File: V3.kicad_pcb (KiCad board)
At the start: 2 copper layers, 164.6 x 93.3 mm, 73 parts, among them IC1 MCP4451-103E_ST, IC2 MCP4451-103E_ST, IC3 MCP4451-103E_ST, IC4 MCP4451-103E_ST, IC5 MCP4451-103E_ST, IC6 MCP4451-103E_ST, J1 Barrel_Jack, J2 Conn_01x22_Female, U1 AMPLIFIER-PAM8403, U10 AMPLIFIER-PAM8403, U11 AMPLIFIER-PAM8403, U12 AMPLIFIER-PAM8403, U2 AMPLIFIER-PAM8403, U3 AMPLIFIER-PAM8403, U4 AMPLIFIER-PAM8403, U5 AMPLIFIER-PAM8403, U6 AMPLIFIER-PAM8403, U7 AMPLIFIER-PAM8403, U8 AMPLIFIER-PAM8403, U9 AMPLIFIER-PAM8403

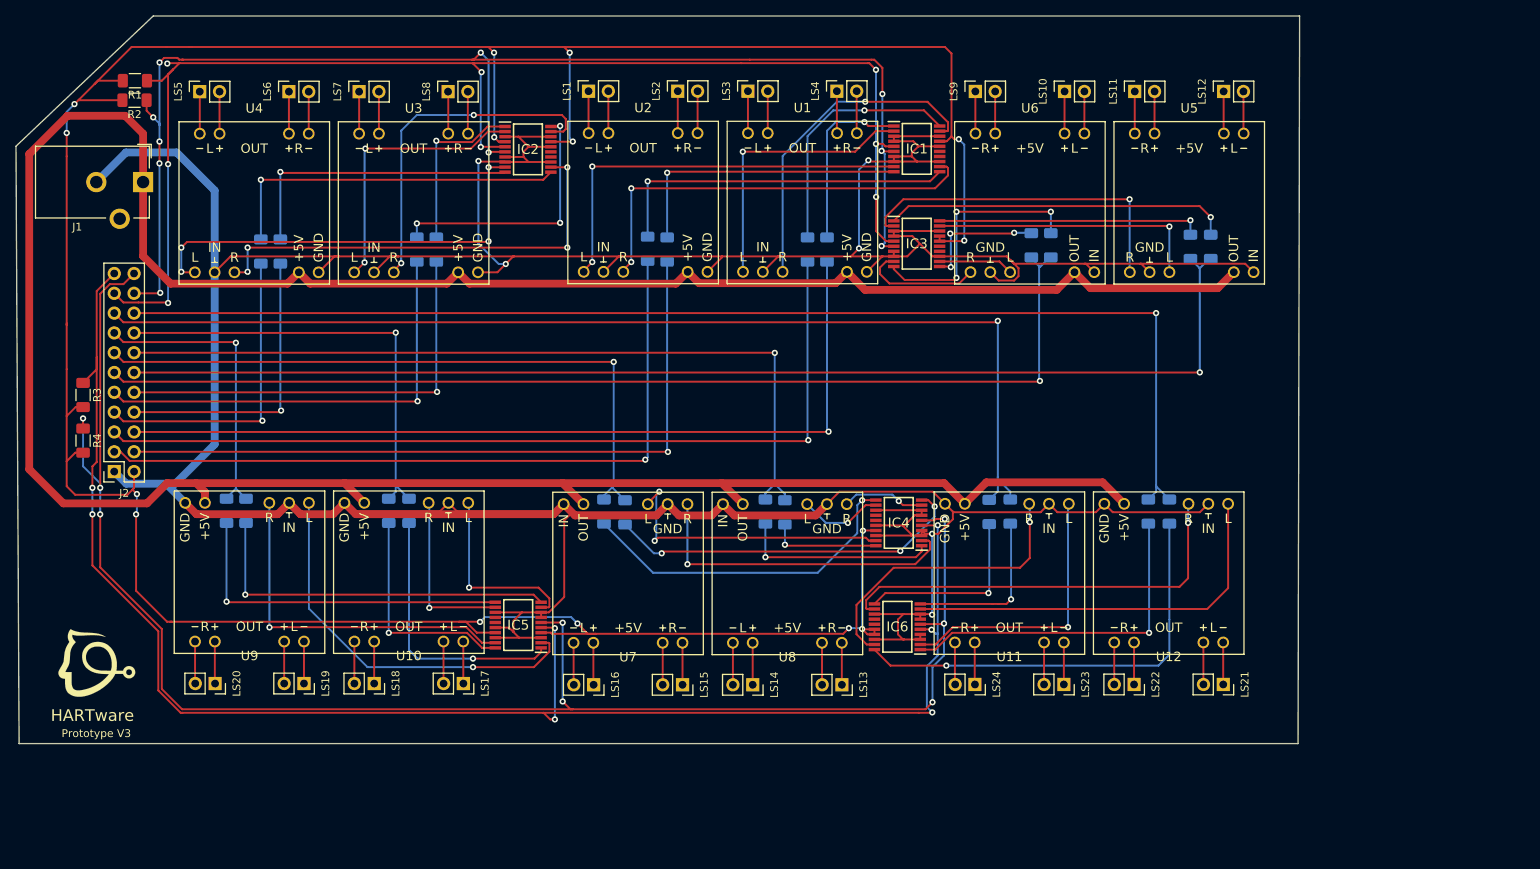
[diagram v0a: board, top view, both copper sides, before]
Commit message: Release V3.0.1
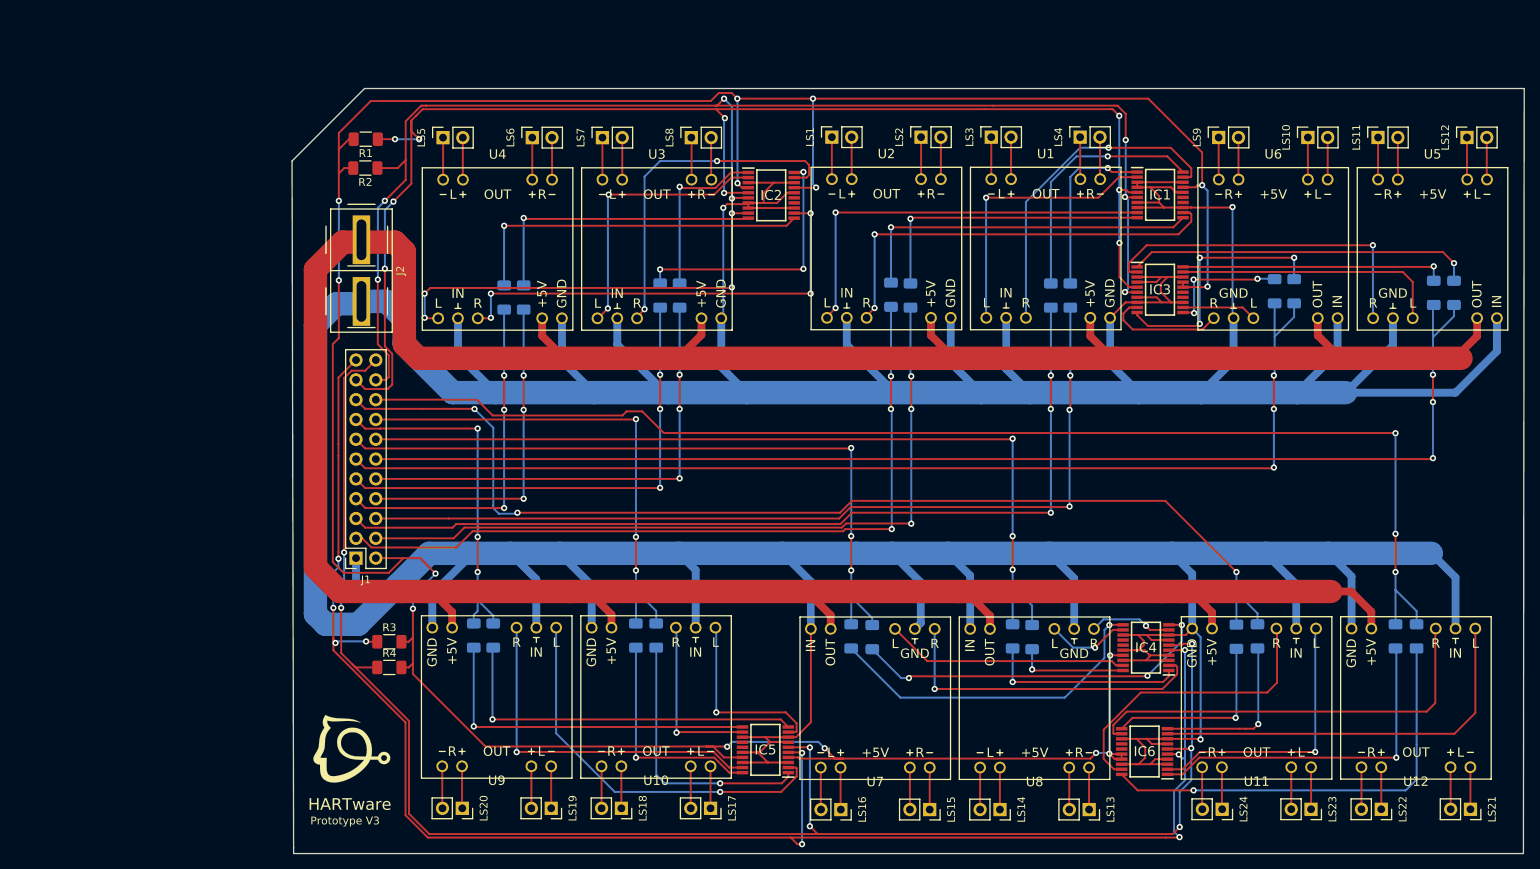
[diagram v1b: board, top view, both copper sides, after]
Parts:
- J1: value Barrel_Jack -> Conn_01x22_Female; footprint Barrel Jack:BarrelJack_CUI_PJ-102AH_Horizontal -> Pin Socket 2.54mm:PinSocket_2x11_P2.54mm_Vertical
- J2: value Conn_01x22_Female -> PowerPole; footprint Pin Socket 2.54mm:PinSocket_2x11_P2.54mm_Vertical -> PowerPole:45A-VERT-PAIR
- moved J1 55.4 mm to (128.8, 118.9), turned to 180 degrees
- moved R3 50.4 mm to (133.1, 129.6), turned to 0 degrees
- moved R4 48.9 mm to (133.1, 132.9), turned to 0 degrees
- moved J2 40.9 mm to (129.5, 82.0), turned to 270 degrees
- moved IC5 35.5 mm to (181.3, 143.5)
- moved LS14 35.5 mm to (211.4, 151.2)
- moved LS15 35.5 mm to (202.4, 151.2)
- moved LS17 35.5 mm to (174.3, 151.0)
- moved LS18 35.5 mm to (162.8, 151.0)
- moved LS19 35.5 mm to (153.8, 151.0)
- moved LS23 35.5 mm to (251.3, 151.1)
- moved LS24 35.5 mm to (239.9, 151.1)
- moved R21 35.5 mm to (167.3, 128.8)
- moved U11 35.5 mm to (244.3, 136.8)
- moved U7 35.5 mm to (195.4, 136.9)
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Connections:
- J1 pad 1: VDD -> GND
- J1 pad 2: GND -> TeensyVDD
- J1 pad 3: (no net) -> FREQ1
- J2 pad 1: GND -> VDD
- J2 pad 2: TeensyVDD -> GND
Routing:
- net GND: track 624.1 -> 837.5 mm, vias 6 -> 3
- net VDD: track 388.2 -> 418.0 mm
- net FREQ12: track 104.1 -> 111.5 mm, vias 1 -> 3
- net FREQ9: track 137.6 -> 144.9 mm, vias 1 -> 3
- net FREQ10: track 153.6 -> 160.9 mm, vias 1 -> 3
- net SCL1: track 207.7 -> 214.8 mm, vias 7 -> 9
- net FREQ14: track 57.9 -> 64.9 mm, vias 1 -> 3
- net SCL0: track 174.4 -> 181.2 mm, vias 8 -> 9
- net FREQ11: track 85.1 -> 91.8 mm, vias 1 -> 3
- net FREQ13: track 38.5 -> 45.2 mm, vias 1 -> 3
- net Net-(IC4-Pad19): track 37.4 -> 31.3 mm, vias 2 -> 0
- net FREQ6: track 38.0 -> 43.4 mm, vias 1 -> 3
- net FREQ8: track 55.8 -> 61.0 mm, vias 1 -> 3
- net FREQ7: track 57.5 -> 62.7 mm, vias 1 -> 3
- net FREQ5: track 40.0 -> 45.2 mm, vias 1 -> 3
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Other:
- board size 164.6 x 93.3 mm -> 158 x 98.1 mm
